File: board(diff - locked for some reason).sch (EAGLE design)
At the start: 21 parts, among them IC1 ATMEGA644-20PU, J2 2468, J3 2468, Q1 2N3906, T1 2N3904, T2 2N3904, T3 2N3904, T4 2N3904, U1 MCP1825S-3302E/DB

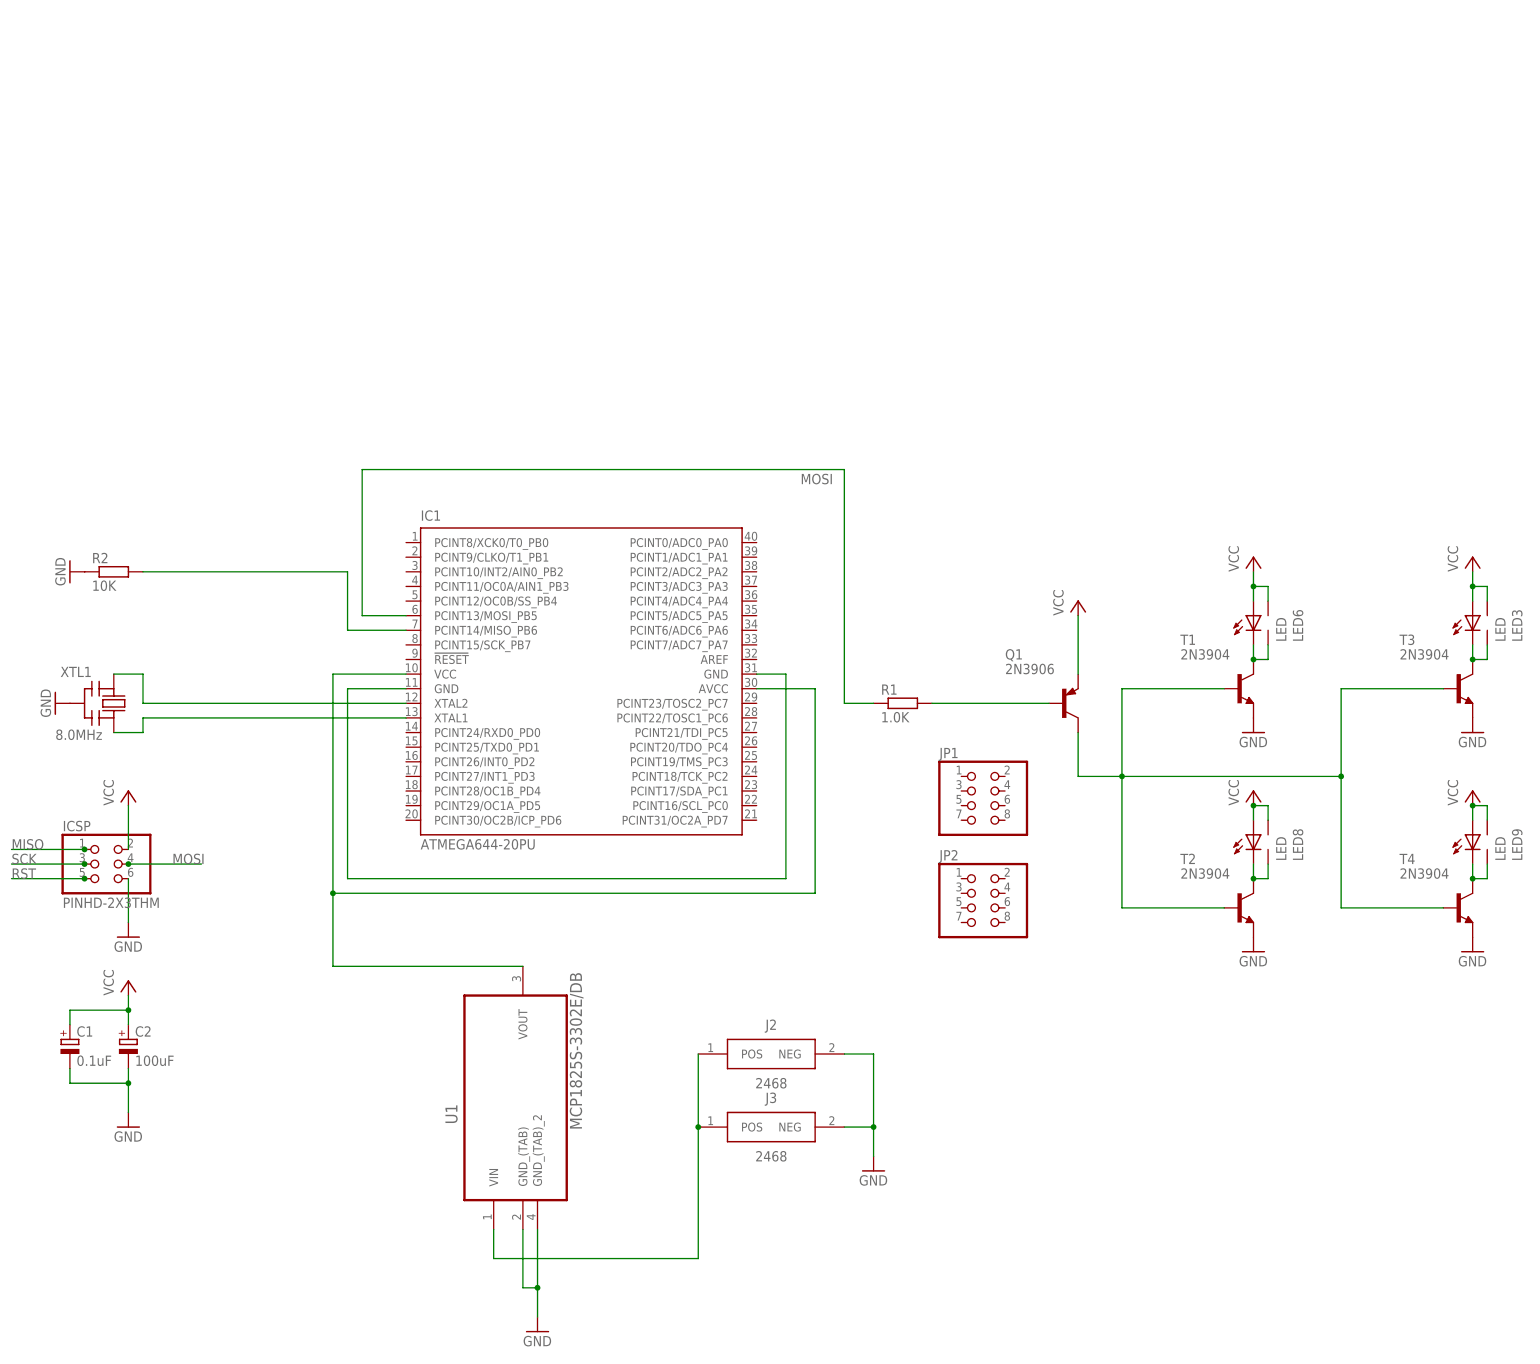
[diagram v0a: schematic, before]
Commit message: modified board
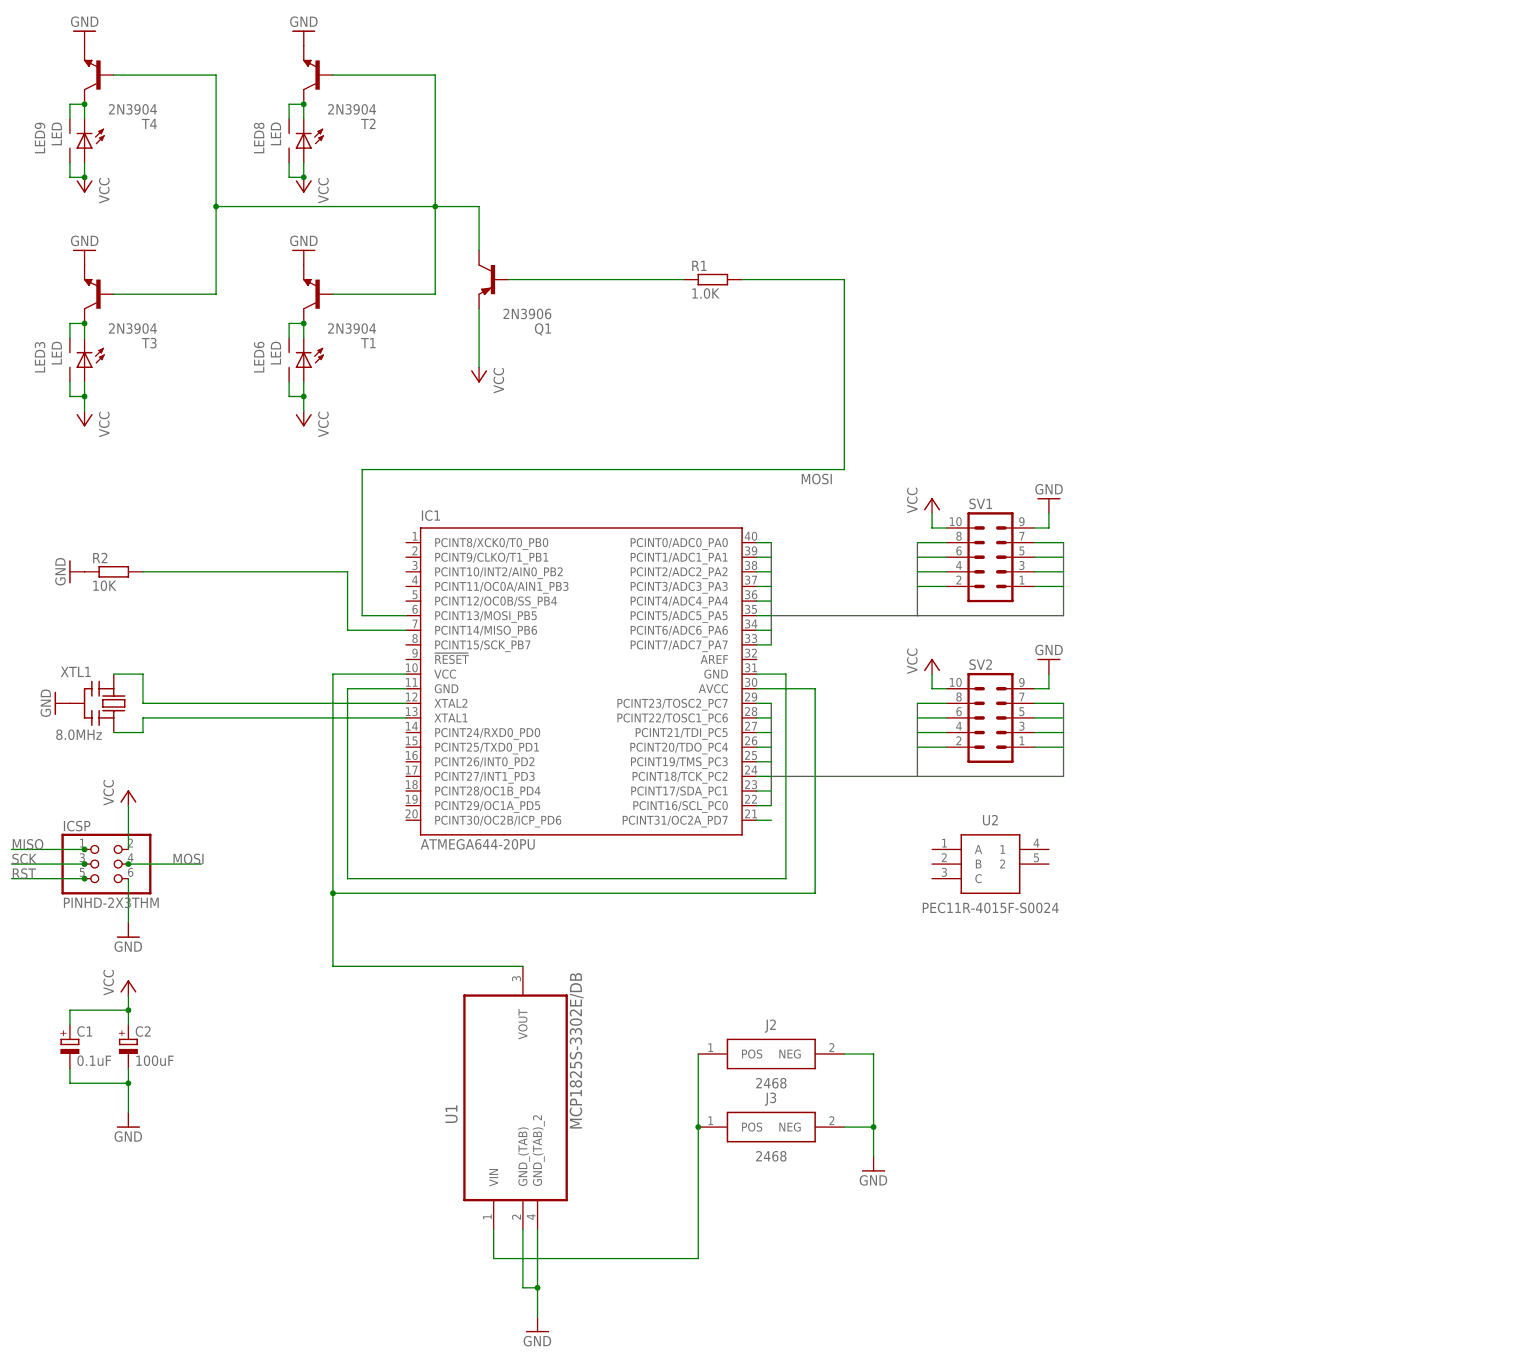
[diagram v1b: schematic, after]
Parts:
- removed JP1, JP2: (no value), pinhead:PINHD-2X4
- added SV1, SV2: (no value), con-lstb:MA05-2
- added U2: PEC11R-4015F-S0024, SamacSys_Parts:PEC11R-4015F-S0024
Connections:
- removed net N$7: Q1.B, R1.2
- new net N$21: IC1.PCINT31/OC2A_PD7
- new net N$22: Q1.B, R1.1
- new net PA0: IC1.PCINT0/ADC0_PA0, SV1.8
- new net PA1: IC1.PCINT1/ADC1_PA1, SV1.6
- new net PA2: IC1.PCINT2/ADC2_PA2, SV1.4
- new net PA3: IC1.PCINT3/ADC3_PA3, SV1.2
- new net PA4: IC1.PCINT4/ADC4_PA4, SV1.1
- new net PA5: IC1.PCINT5/ADC5_PA5, SV1.3
- new net PA6: IC1.PCINT6/ADC6_PA6, SV1.5
- new net PA7: IC1.PCINT7/ADC7_PA7, SV1.7
- new net PC0: IC1.PCINT16/SCL_PC0, SV2.8
- new net PC1: IC1.PCINT17/SDA_PC1, SV2.6
- new net PC2: IC1.PCINT18/TCK_PC2, SV2.4
- new net PC3: IC1.PCINT19/TMS_PC3, SV2.2
- new net PC4: IC1.PCINT20/TDO_PC4, SV2.1
- new net PC5: IC1.PCINT21/TDI_PC5, SV2.3
- new net PC6: IC1.PCINT22/TOSC1_PC6, SV2.5
- new net PC7: IC1.PCINT23/TOSC2_PC7, SV2.7
- net GND: now also SV1.9, SV2.9
- net MOSI: now also R1.2; no longer R1.1
- net VCC: now also SV1.10, SV2.10
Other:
- moved on the sheet: LED3, LED6, LED8, LED9, Q1, R1, T1, T2, T3, T4
